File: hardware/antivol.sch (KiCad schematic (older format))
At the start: 38 parts, among them J1 Conn_01x02, J2 Conn_01x06, J3 Conn_01x02, Q1 AO3401A, Q2 AO3401A, Q3 AO3401A, U1 ESP-WROOM-32, U2 TP4054, U3 ME6211C33, U4 KXTJ3-1057

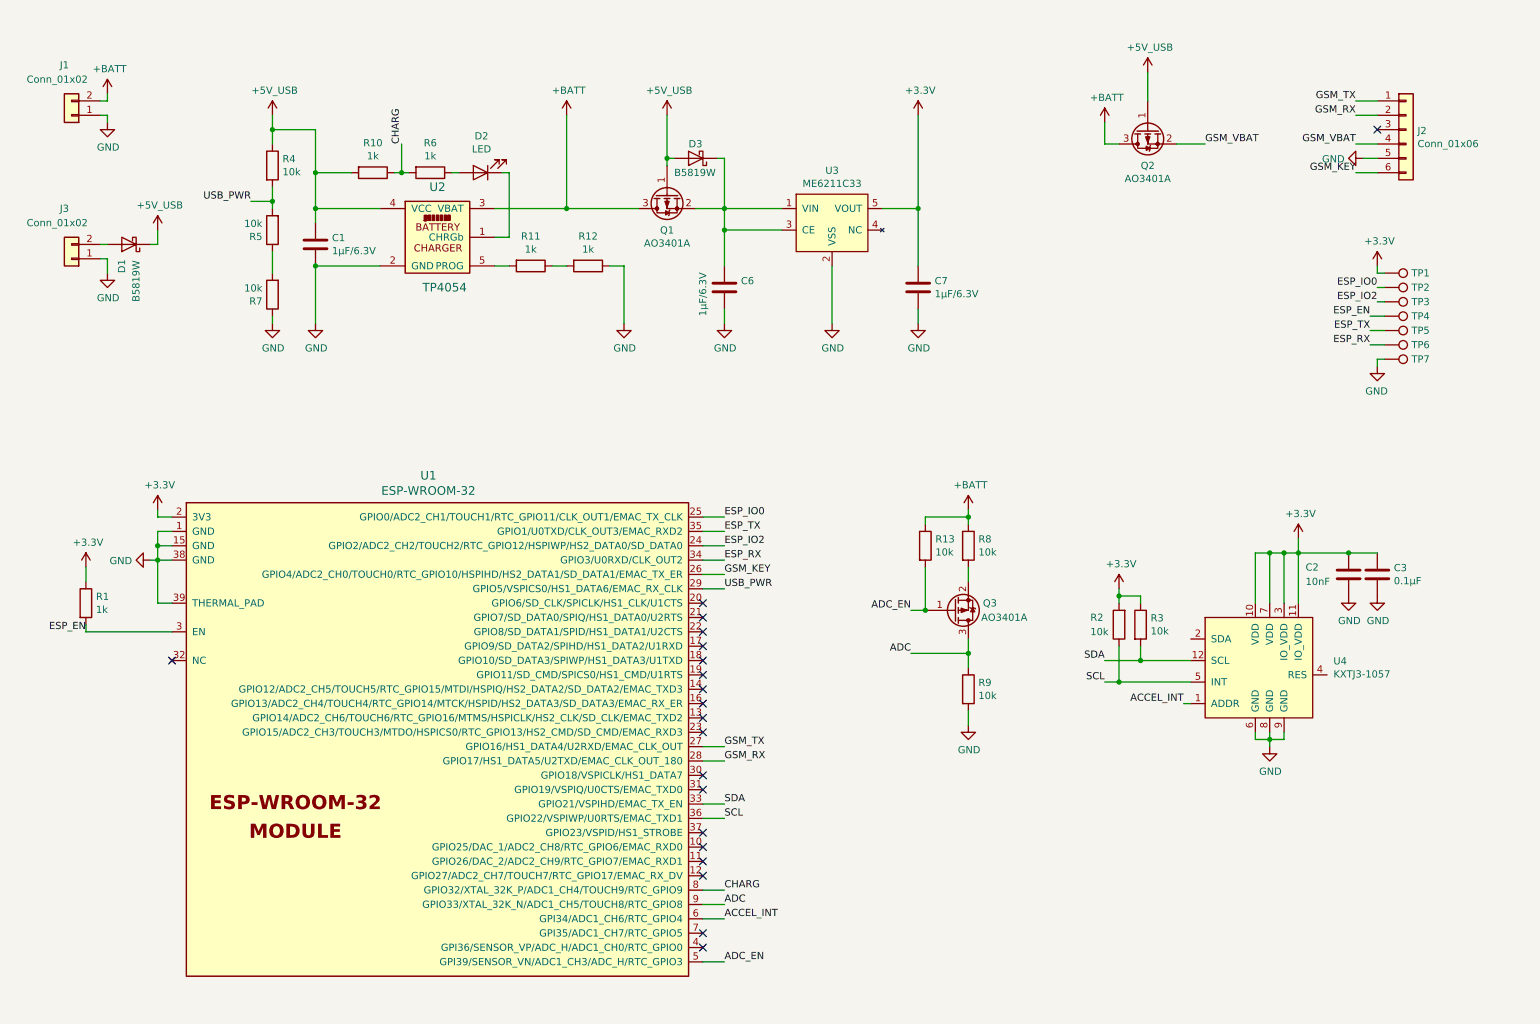
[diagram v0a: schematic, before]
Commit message: cp2102
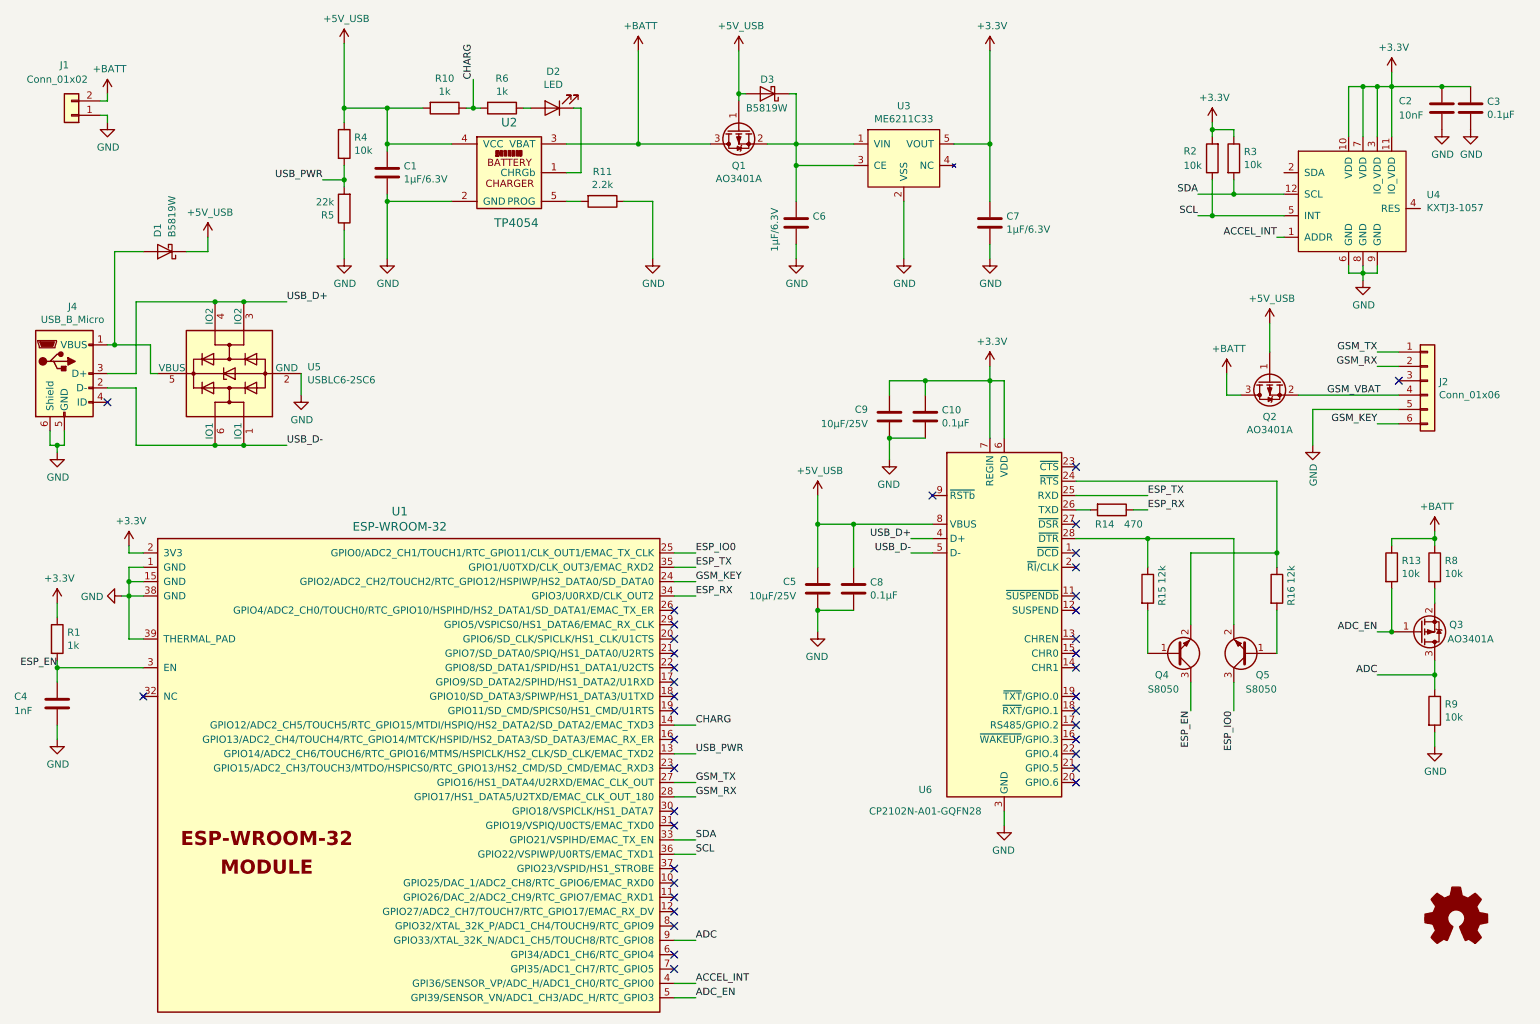
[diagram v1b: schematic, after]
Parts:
- removed J3: Conn_01x02, Connector_PinHeader_2.54mm:PinHeader_1x02_P2.54mm_Vertical, symbol Connector_Generic:Conn_01x02
- removed R12: 1k, Resistor_SMD:R_0603_1608Metric, symbol Device:R
- removed R7: 10k, Resistor_SMD:R_0603_1608Metric, symbol Device:R
- removed TP1, TP2, TP3, TP4, TP5, TP6, TP7: TestPoint, TestPoint:TestPoint_Pad_D1.5mm, symbol Connector:TestPoint
- added C10, C8: 0.1µF, Capacitor_SMD:C_0603_1608Metric, symbol Device:C
- added C4: 1nF, Capacitor_SMD:C_0603_1608Metric, symbol Device:C
- added C5, C9: 10µF/25V, Capacitor_SMD:C_0805_2012Metric, symbol Device:C
- added J4: USB_B_Micro, Connector_USB:USB_Micro-B_Molex-105017-0001, symbol Connector:USB_B_Micro
- added Q4, Q5: S8050, Package_TO_SOT_SMD:SOT-23, symbol Device:Q_NPN_BEC
- added R14: 470, Resistor_SMD:R_0603_1608Metric, symbol Device:R
- added R15, R16: 12k, Resistor_SMD:R_0603_1608Metric, symbol Device:R
- added U5: USBLC6-2SC6, Package_TO_SOT_SMD:SOT-23-6_Handsoldering, symbol Power_Protection:USBLC6-2SC6
- added U6: CP2102N-A01-GQFN28, Package_DFN_QFN:QFN-28-1EP_5x5mm_P0.5mm_EP3.35x3.35mm, symbol Interface_USB:CP2102N-A01-GQFN28
- R11: value 1k -> 2.2k; LCSC C21190 -> C4190
- R5: value 10k -> 22k; LCSC C25804 -> C31850
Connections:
- net ESP_IO2 is gone; now on net GSM_KEY: U1.24 (GPIO2/ADC2_CH2/TOUCH2/RTC_GPIO12/HSPIWP/HS2_DATA0/SD_DATA0)
- net +3V3: now also C10.1, C9.2, U6.6 (VDD), U6.7 (REGIN)
- net +5V_USB: now also C5.2, C8.1, U6.8 (VBUS)
- net ACCEL_INT: now also U1.4 (GPI36/SENSOR_VP/ADC_H/ADC1_CH0/RTC_GPIO0); no longer U1.6 (GPI34/ADC1_CH6/RTC_GPIO4)
- net CHARG: now also U1.14 (GPIO12/ADC2_CH5/TOUCH5/RTC_GPIO15/MTDI/HSPIQ/HS2_DATA2/SD_DATA2/EMAC_TXD3); no longer U1.8 (GPIO32/XTAL_32K_P/ADC1_CH4/TOUCH9/RTC_GPIO9)
- net ESP_EN: now also C4.2, Q4.3 (C)
- net ESP_IO0: now also Q5.3 (C)
- net ESP_RX: now also R14.1
- net ESP_TX: now also U6.25 (RXD)
- net GND: now also R11.1, R5.1, C10.2, C4.1, C5.1, C8.2, C9.1, J4.5 (GND), J4.6 (Shield), U5.2 (GND), U6.29 (GND), U6.3 (GND)
- net GSM_KEY: no longer U1.26 (GPIO4/ADC2_CH0/TOUCH0/RTC_GPIO10/HSPIHD/HS2_DATA1/SD_DATA1/EMAC_TX_ER)
- net USB_PWR: now also U1.13 (GPIO14/ADC2_CH6/TOUCH6/RTC_GPIO16/MTMS/HSPICLK/HS2_CLK/SD_CLK/EMAC_TXD2); no longer U1.29 (GPIO5/VSPICS0/HS1_DATA6/EMAC_RX_CLK)
- net at D1.2 (A): now also J4.1 (VBUS), U5.5 (VBUS)
- new net: Q4.2 (E), R16.1, U6.24 (~RTS)
- new net: R14.2, U6.26 (TXD)
- new net: Q5.2 (E), R15.1, U6.28 (~DTR)
- new net: Q5.1 (B), R16.2
- new net: Q4.1 (B), R15.2
- new net USB_D+: J4.3 (D+), U5.3 (IO2), U5.4 (IO2), U6.4 (D+)
- new net USB_D-: J4.2 (D-), U5.1 (IO1), U5.6 (IO1), U6.5 (D-)
- no-connect marks 20 -> 39
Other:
- moved on the sheet: C1, C2, C3, C6, C7, D1, D2, D3, J2, Q1, Q2, Q3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

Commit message: v1
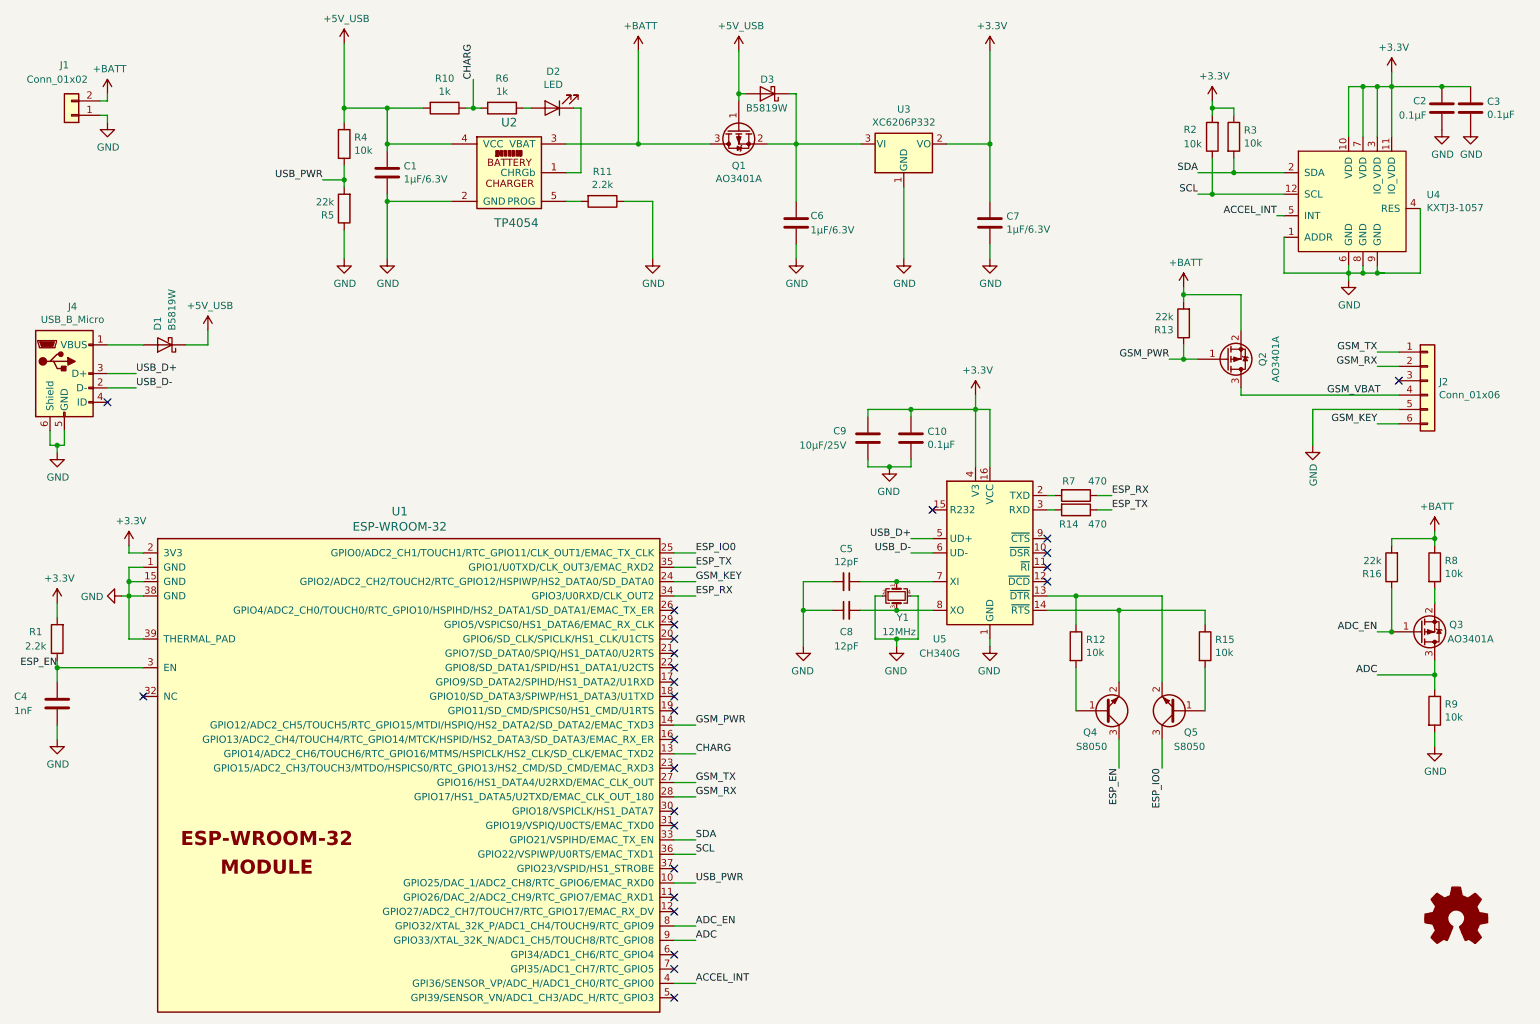
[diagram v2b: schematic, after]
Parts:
- removed C5: 10µF/25V, Capacitor_SMD:C_0805_2012Metric, symbol Device:C
- removed C8: 0.1µF, Capacitor_SMD:C_0603_1608Metric, symbol Device:C
- removed U3: ME6211C33, Package_TO_SOT_SMD:SOT-23-5, symbol components:ME6211C33
- removed U5: USBLC6-2SC6, Package_TO_SOT_SMD:SOT-23-6_Handsoldering, symbol Power_Protection:USBLC6-2SC6
- removed U6: CP2102N-A01-GQFN28, Package_DFN_QFN:QFN-28-1EP_5x5mm_P0.5mm_EP3.35x3.35mm, symbol Interface_USB:CP2102N-A01-GQFN28
- added C5, C8: 12pF, Capacitor_SMD:C_0603_1608Metric, symbol Device:C_Small
- added R12: 10k, Resistor_SMD:R_0603_1608Metric, symbol Device:R
- added R7: 470, Resistor_SMD:R_0603_1608Metric, symbol Device:R
- added U3: XC6206P332, Package_TO_SOT_SMD:SOT-23, symbol Regulator_Linear:AP1117-33
- added U5: CH340G, Package_SO:SOIC-16_3.9x9.9mm_P1.27mm, symbol Interface_USB:CH340G
- added Y1: 12MHz, Crystal:Crystal_SMD_3225-4Pin_3.2x2.5mm, symbol Device:Crystal_GND24_Small
- C2: value 10nF -> 0.1µF; LCSC C57112 -> C14663
- R1: value 1k -> 2.2k; LCSC C21190 -> C4190
- R13: value 10k -> 22k; LCSC C25804 -> C31850
- R15: value 12k -> 10k; LCSC C22790 -> C25804
- R16: value 12k -> 22k; LCSC C22790 -> C31850
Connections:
- net +3V3: now also R1.2, U3.2 (VO), U5.16 (VCC), U5.4 (V3); no longer R1.1
- net +5V_USB: no longer Q2.1 (G)
- net +BATT: now also Q2.2 (S), R13.2, R16.2; no longer Q2.3 (D), R13.1
- net ACCEL_INT: now also U4.5 (INT); no longer U4.1 (ADDR)
- net ADC_EN: now also R16.1, U1.8 (GPIO32/XTAL_32K_P/ADC1_CH4/TOUCH9/RTC_GPIO9); no longer R13.2, U1.5 (GPI39/SENSOR_VN/ADC1_CH3/ADC_H/RTC_GPIO3)
- net CHARG: now also U1.13 (GPIO14/ADC2_CH6/TOUCH6/RTC_GPIO16/MTMS/HSPICLK/HS2_CLK/SD_CLK/EMAC_TXD2); no longer U1.14 (GPIO12/ADC2_CH5/TOUCH5/RTC_GPIO15/MTDI/HSPIQ/HS2_DATA2/SD_DATA2/EMAC_TXD3)
- net ESP_EN: now also R1.1; no longer R1.2
- net ESP_RX: now also R7.1; no longer R14.1
- net ESP_TX: now also R14.1
- net GND: now also U4.1 (ADDR), U4.4 (RES), C5.2, C8.1, U3.1 (GND), U5.1 (GND), Y1.2, Y1.4
- net GSM_VBAT: now also Q2.3 (D); no longer Q2.2 (S)
- net SCL: now also U4.12 (SCL); no longer U4.5 (INT)
- net SDA: now also U4.2 (SDA); no longer U4.12 (SCL)
- net USB_D+: now also U5.5 (UD+)
- net USB_D-: now also U5.6 (UD-)
- net USB_PWR: now also U1.10 (GPIO25/DAC_1/ADC2_CH8/RTC_GPIO6/EMAC_RXD0); no longer U1.13 (GPIO14/ADC2_CH6/TOUCH6/RTC_GPIO16/MTMS/HSPICLK/HS2_CLK/SD_CLK/EMAC_TXD2)
- net at C6.1, D3.1 (K), Q1.2 (S): now also U3.3 (VI)
- net at Q4.2 (E): now also R15.1, U5.14 (~RTS); no longer R16.1
- net at R14.2: now also U5.3 (RXD)
- net at Q5.2 (E): now also R12.1, U5.13 (~DTR); no longer R15.1
- net at Q5.1 (B): now also R15.2; no longer R16.2
- net at Q4.1 (B): now also R12.2; no longer R15.2
- new net: R7.2, U5.2 (TXD)
- new net: C5.1, U5.7 (XI), Y1.1
- new net: C8.2, U5.8 (XO), Y1.3
- new net GSM_PWR: Q2.1 (G), R13.1, U1.14 (GPIO12/ADC2_CH5/TOUCH5/RTC_GPIO15/MTDI/HSPIQ/HS2_DATA2/SD_DATA2/EMAC_TXD3)
- no-connect marks 39 -> 26
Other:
- moved on the sheet: C10, C9, D1, Q4, Q5, R14, R2, R3
